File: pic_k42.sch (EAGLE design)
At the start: 88 parts, among them IC1 PIC18F57K42-E_PT, IC2 REF3440IDBVR, IC3 MAX232, IC4 ILAMP, J1 MLE-105-01-G-DV, K1 G6K-2P, P10_V 10 volts, Q1 ASF1, U1 LM78L05ACMX/NOPB, X1 RX-2, X10 J1, X11 22-23-2021, X2 TX-2, X3 RESETJMP, X4 MINI-USB-UX60A-MB-5ST, X5 PORTA, X6 PORTD, X7 PORTB, X8 J3, X9 J2

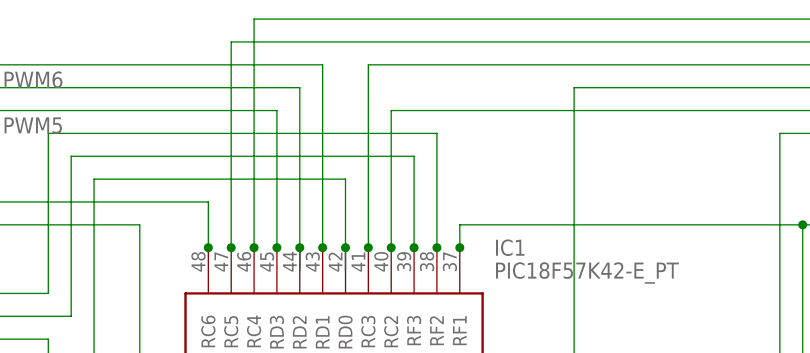
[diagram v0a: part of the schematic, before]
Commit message: up
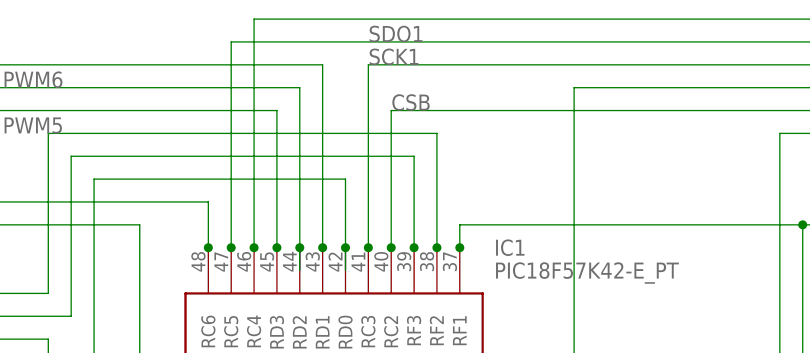
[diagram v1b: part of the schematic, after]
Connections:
- net N$30 renamed SDO1
- net N$31 renamed SCK1
- net N$33 renamed CSB
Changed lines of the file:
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@@
 </segment>
 </net>
-<net name="N$30" class="0">
+<net name="SDO1" class="0">
 <segment>
 <pinref part="IC1" gate="G$1" pin="RC5"/>
@@
 <junction x="142.24" y="83.82"/>
 <junction x="43.18" y="88.9"/>
+<label x="58.42" y="111.76" size="1.778" layer="95"/>
 </segment>
 </net>
-<net name="N$31" class="0">
+<net name="SCK1" class="0">
 <segment>
 <pinref part="IC1" gate="G$1" pin="RC3"/>
@@
 <junction x="142.24" y="81.28"/>
 <junction x="58.42" y="88.9"/>
+<label x="58.42" y="109.22" size="1.778" layer="95"/>
 </segment>
 </net>
@@
 </segment>
 </net>
-<net name="N$33" class="0">
+<net name="CSB" class="0">
 <segment>
 <pinref part="IC1" gate="G$1" pin="RC2"/>
@@
 <junction x="142.24" y="76.2"/>
 <junction x="60.96" y="88.9"/>
+<label x="60.96" y="104.14" size="1.778" layer="95"/>
 </segment>
 </net>

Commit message: Revert "up"
This reverts commit 2af174bc1ac14fa5ed8294ec6c26e2dbc3c0e6fd.
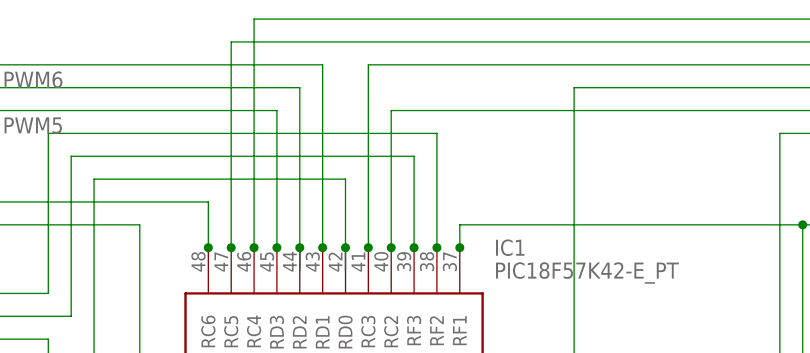
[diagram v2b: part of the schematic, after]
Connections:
- net CSB renamed N$33
- net SCK1 renamed N$31
- net SDO1 renamed N$30
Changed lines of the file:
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@@
 </segment>
 </net>
-<net name="SDO1" class="0">
+<net name="N$30" class="0">
 <segment>
 <pinref part="IC1" gate="G$1" pin="RC5"/>
@@
 <junction x="142.24" y="83.82"/>
 <junction x="43.18" y="88.9"/>
-<label x="58.42" y="111.76" size="1.778" layer="95"/>
 </segment>
 </net>
-<net name="SCK1" class="0">
+<net name="N$31" class="0">
 <segment>
 <pinref part="IC1" gate="G$1" pin="RC3"/>
@@
 <junction x="142.24" y="81.28"/>
 <junction x="58.42" y="88.9"/>
-<label x="58.42" y="109.22" size="1.778" layer="95"/>
 </segment>
 </net>
@@
 </segment>
 </net>
-<net name="CSB" class="0">
+<net name="N$33" class="0">
 <segment>
 <pinref part="IC1" gate="G$1" pin="RC2"/>
@@
 <junction x="142.24" y="76.2"/>
 <junction x="60.96" y="88.9"/>
-<label x="60.96" y="104.14" size="1.778" layer="95"/>
 </segment>
 </net>
